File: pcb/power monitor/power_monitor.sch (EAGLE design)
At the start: 23 parts

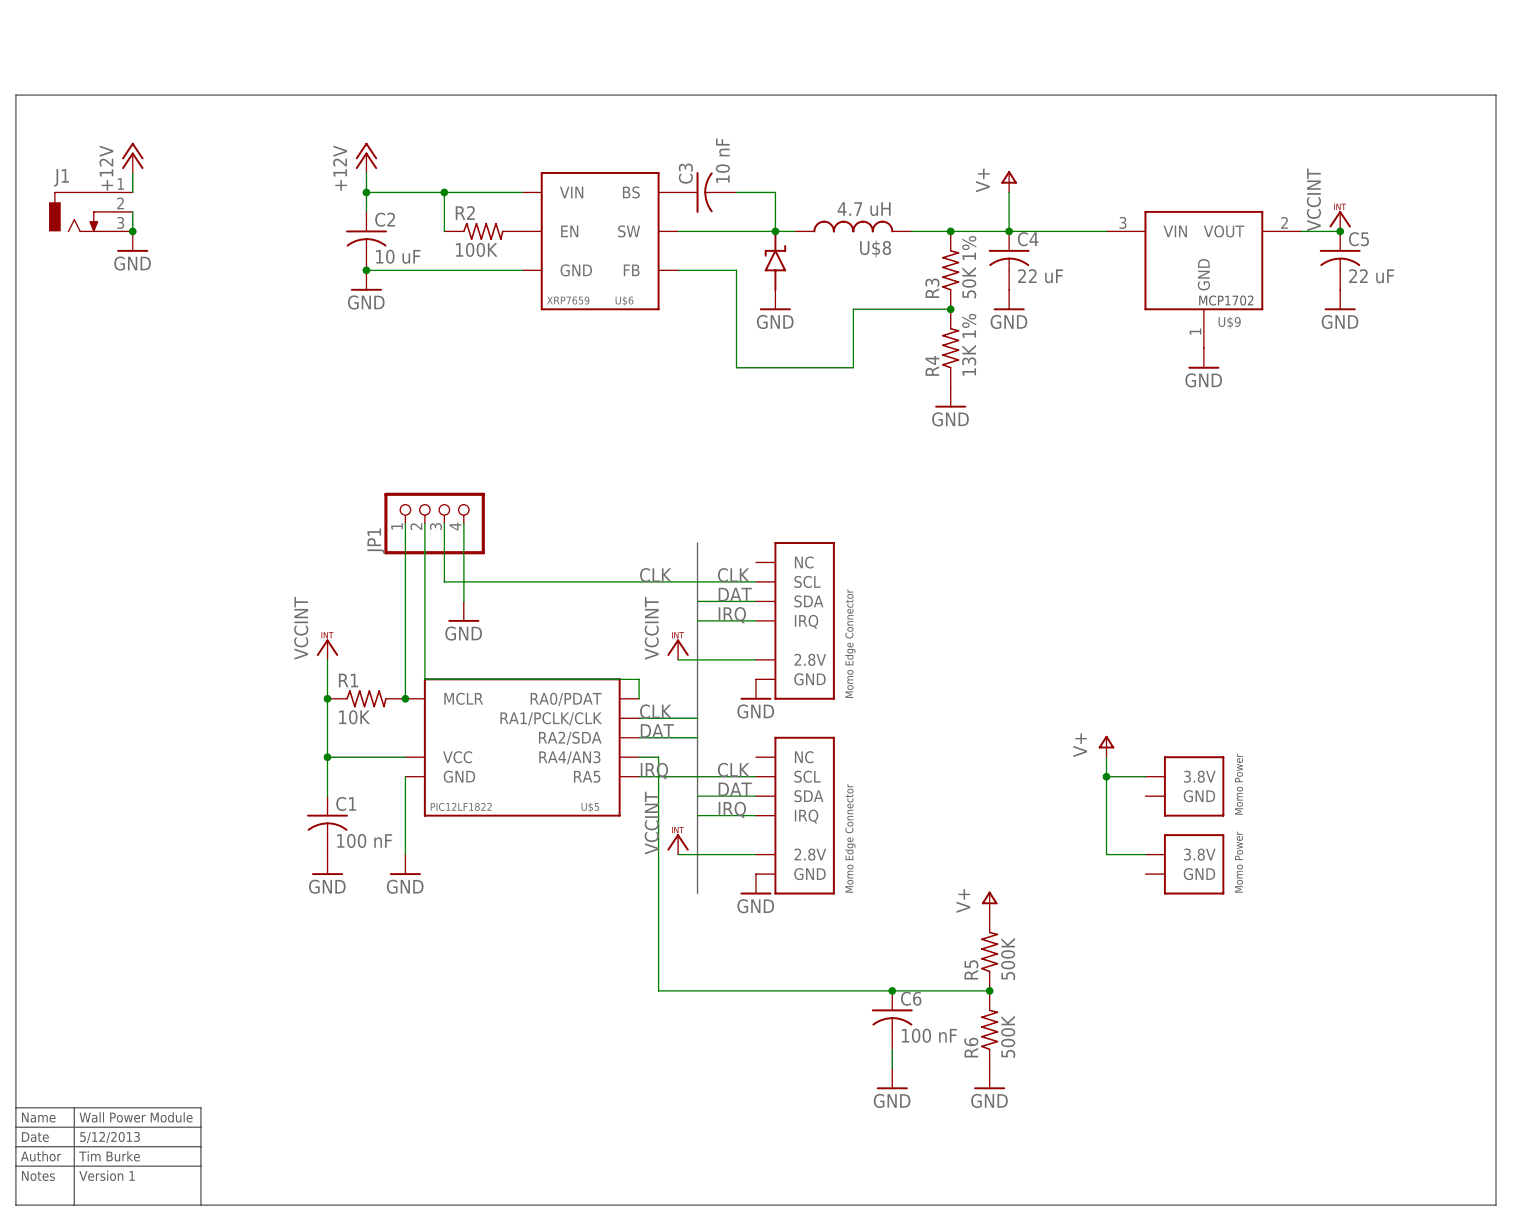
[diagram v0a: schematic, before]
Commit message: Signed-off-by: timcronin <tmpcronin@gmail.com>
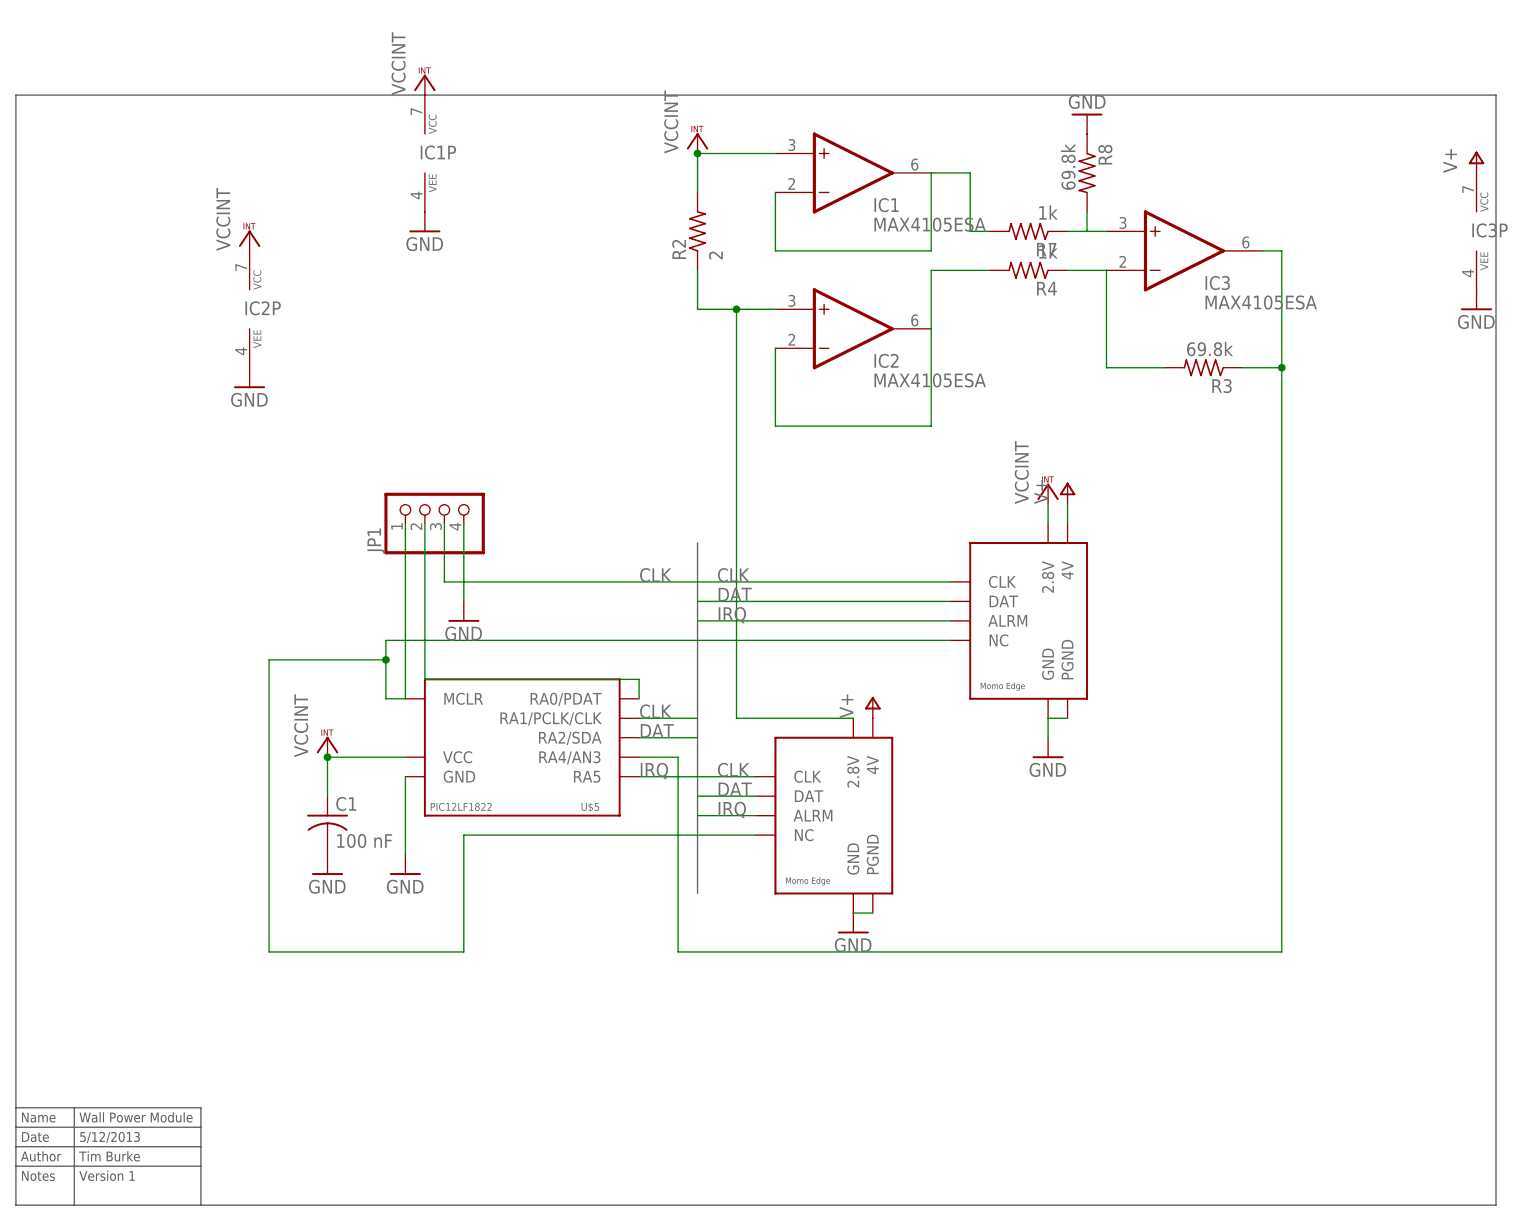
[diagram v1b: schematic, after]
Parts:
- removed C2: 10 uF, rcl:C-USC0805
- removed C3: 10 nF, rcl:C-USC0402
- removed C4: 22 uF, rcl:C-USC1206
- removed C5: 22 uF, rcl:C-USC0402
- removed C6: 100 nF, rcl:C-USC0402
- removed J1: (no value), con-jack:DCJ0303
- removed R1: 10K, rcl:R-US_R0603
- removed R5, R6: 500K, rcl:R-US_R0603
- removed U$1: MOMO-EDGE-SMALL-M, components:MOMO-EDGE-SMALL-M
- removed U$2: MOMO-EDGE-SMALL-F, components:MOMO-EDGE-SMALL-F
- removed U$3: MOMO-EDGE-POWER-M, components:MOMO-EDGE-POWER-M
- removed U$4: MOMO-EDGE-POWER-F, components:MOMO-EDGE-POWER-F
- removed U$8: 4.7 uH, components:NR6028-INDUCTOR
- removed U$9: MCP1702, components:MCP1702
- added IC1, IC2, IC3: MAX4105ESA, maxim:MAX4105ESA
- added R7: 1k, rcl:R-US_R0603
- added R8: 69.8k, rcl:R-US_R0603
- R2: value 100K -> 2
- R3: value 50K 1% -> 69.8k
- R4: value 13K 1% -> 1k
- U$6: value XRP7659 -> MOMO-EDGE-8F; device components:XRP7659 -> components:MOMO-EDGE-8F
- U$7: value DIODE_SS2P3 -> MOMO-EDGE-8M; device components:DIODE_SS2P3 -> components:MOMO-EDGE-8M
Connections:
- removed net +12V: C2.1, J1.1, R2.1, U$6.VIN
- removed net N$5: C6.1, R5.1, R6.2, U$5.RA4/AN3
- removed net N$6: R3.1, R4.2, U$6.FB
- new net N$11: IC2G$1.+IN, R2.1, U$7.2.8V
- new net N$7: IC3G$1.-IN, R3.2, R4.1
- new net N$9: IC3G$1.+IN, R7.1, R8.2
- net CLK: now also U$6.CLK, U$7.CLK; no longer U$1.SCL, U$2.SCL
- net DAT: now also U$6.DAT, U$7.DAT; no longer U$1.SDA, U$2.SDA
- net GND: now also IC1P.VEE, IC2P.VEE, IC3P.VEE, R8.1, U$6.PGND, U$7.GND, U$7.PGND; no longer C2.2, C4.2, C5.2, C6.2, J1.2, J1.3, R4.1, R6.1, U$1.GND, U$2.GND, U$7.AN, U$9.GND
- net IRQ: now also U$6.ALRM, U$7.ALRM; no longer U$1.IRQ, U$2.IRQ
- net N$1: now also U$6.NC, U$7.NC; no longer R1.2
- net N$2: now also IC3G$1.OUT, R3.1, U$5.RA4/AN3; no longer C3.2, U$6.SW, U$7.CATH, U$8.1
- net N$3: now also IC2G$1.-IN, IC2G$1.OUT, R4.2; no longer R2.2, U$6.EN
- net N$4: now also IC1G$1.-IN, IC1G$1.OUT, R7.2; no longer C3.1, U$6.BS
- net V+: now also IC3P.VCC, U$6.4V, U$7.4V; no longer C4.1, R3.2, R5.2, U$3.3.8V, U$4.3.8V, U$8.2, U$9.VIN
- net VCCINT: now also IC1G$1.+IN, IC1P.VCC, IC2P.VCC, R2.2, U$6.2.8V; no longer C5.1, R1.1, U$1.2.8V, U$2.2.8V, U$9.VOUT
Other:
- moved on the sheet: R2, R3, R4
